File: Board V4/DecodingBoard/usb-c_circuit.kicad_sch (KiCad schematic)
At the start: 5 parts, among them J3 USB_C_Receptacle_USB2.0_16P, U3 USBLC6-2SC6

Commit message: footprints updates
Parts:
- J3: footprint UJ20-C-H-G-SMT-1-P16-TR -> Footprints:SAMESKY_UJ20-C-H-G-SMT-1-P16-TR
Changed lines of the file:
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@@
 			)
 		)
-		(property "Footprint" "UJ20-C-H-G-SMT-1-P16-TR"
+		(property "Footprint" "Footprints:SAMESKY_UJ20-C-H-G-SMT-1-P16-TR"
 			(at 44.45 46.99 0)
 			(hide yes)

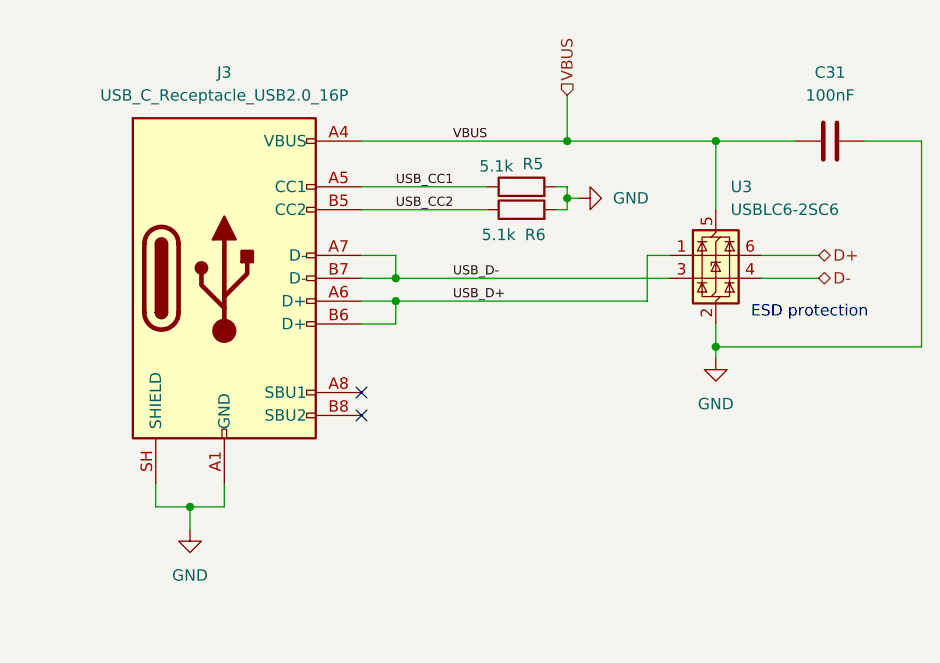
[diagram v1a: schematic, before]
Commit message: First version of the layout
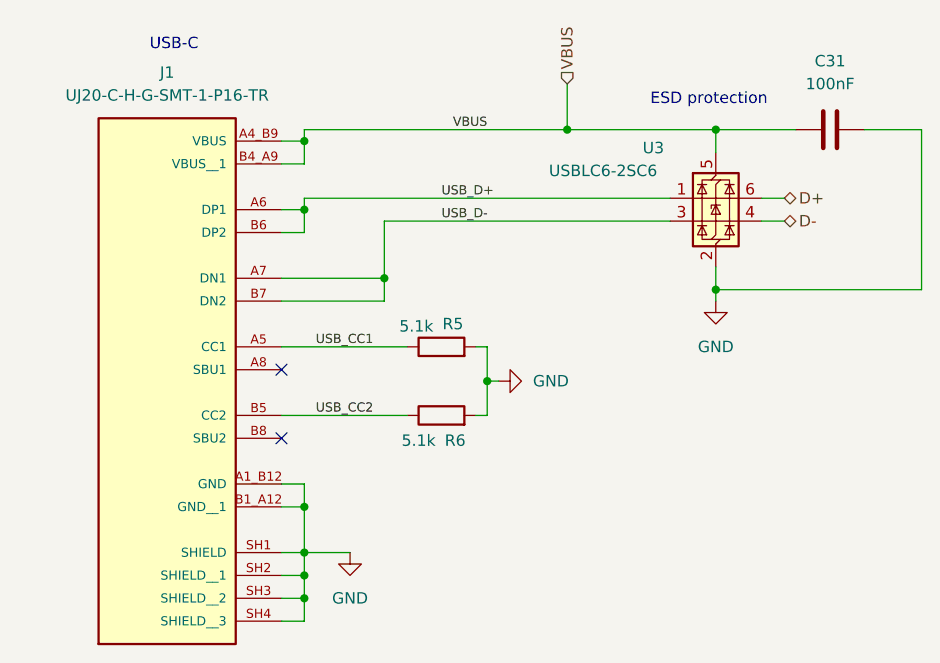
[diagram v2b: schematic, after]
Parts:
- removed J3: USB_C_Receptacle_USB2.0_16P, Footprints:SAMESKY_UJ20-C-H-G-SMT-1-P16-TR, symbol Connector:USB_C_Receptacle_USB2.0_16P
- added J1: UJ20-C-H-G-SMT-1-P16-TR, Footprints:SAMESKY_UJ20-C-H-G-SMT-1-P16-TR, symbol UJ20-C-H-G-SMT-1-P16-TR:UJ20-C-H-G-SMT-1-P16-TR
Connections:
- net GND: now also J1.A1_B12 (GND), J1.B1_A12 (GND__1), J1.SH1 (SHIELD), J1.SH2 (SHIELD__1), J1.SH3 (SHIELD__2), J1.SH4 (SHIELD__3)
- net USB_CC1: now also J1.A5 (CC1)
- net USB_CC2: now also J1.B5 (CC2)
- net USB_D+: now also J1.A6 (DP1), J1.B6 (DP2)
- net USB_D-: now also J1.A7 (DN1), J1.B7 (DN2)
- net VBUS: now also J1.A4_B9 (VBUS), J1.B4_A9 (VBUS__1)
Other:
- note added: "USB-C"
- moved on the sheet: C31, R5, R6, U3
